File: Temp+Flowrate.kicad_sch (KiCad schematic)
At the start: 19 parts, among them Q7 PMOS, Q8 BUK6M61-60PX, U3 TLV9002QDRQ1

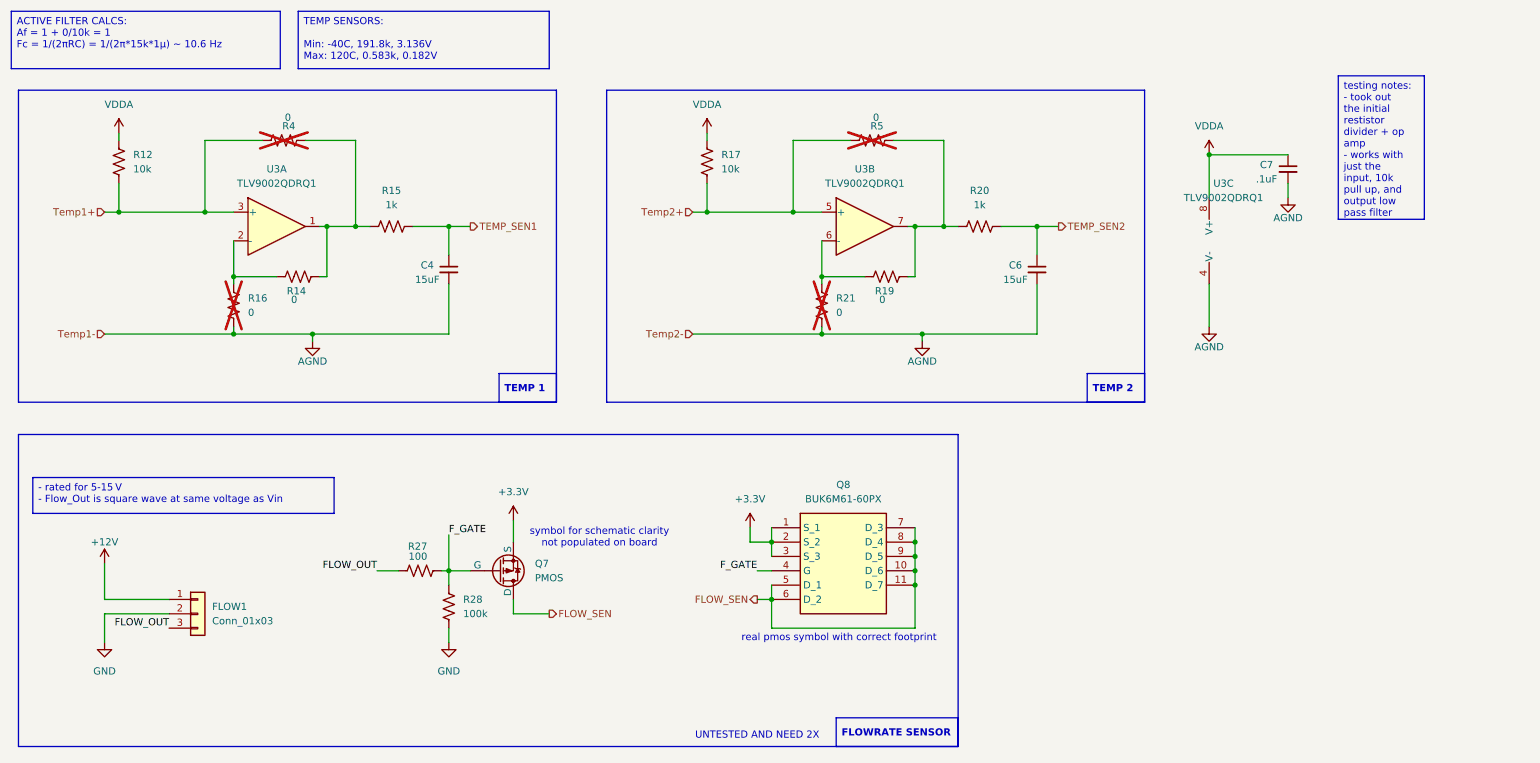
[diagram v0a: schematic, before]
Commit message: schem review changes
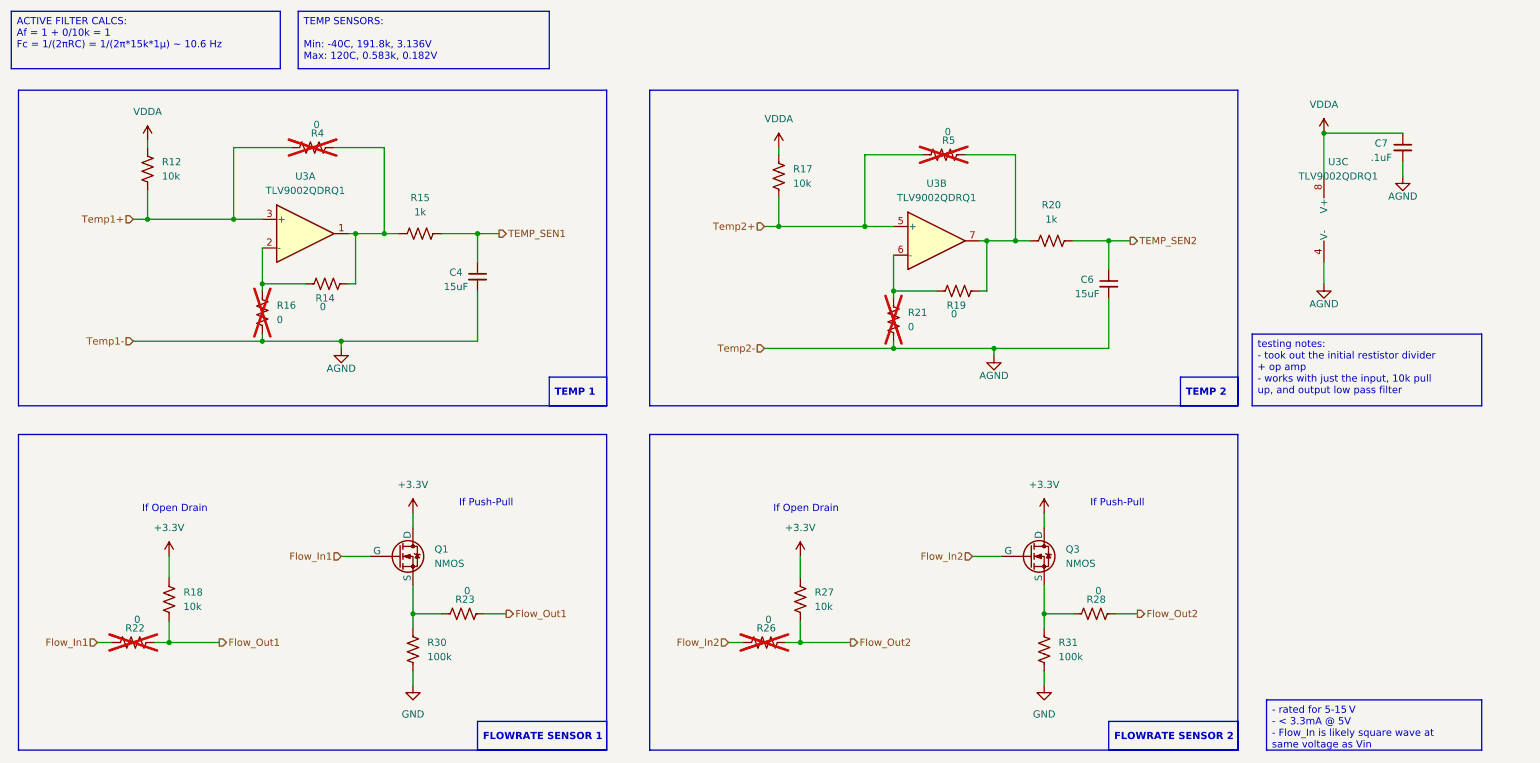
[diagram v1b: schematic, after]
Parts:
- removed FLOW1: Conn_01x03, Connector_Molex:Molex_Nano-Fit_105309-xx03_1x03_P2.50mm_Vertical, symbol Connector_Generic:Conn_01x03
- removed Q7: PMOS, symbol Simulation_SPICE:PMOS
- removed Q8: BUK6M61-60PX, BUK9M34100EX, symbol BUK6M61-60PX:BUK6M61-60PX
- added Q1, Q3: NMOS, IRLML0030TRPBF, symbol Simulation_SPICE:NMOS
- added R18: 10k, Resistor_SMD:R_0603_1608Metric, symbol Device:R_US
- added R22, R23, R26: 0, Resistor_SMD:R_0603_1608Metric, symbol Device:R_US
- added R30, R31: 100k, Resistor_SMD:R_0603_1608Metric, symbol Device:R_US
- R27: value 100 -> 10k
- R28: value 100k -> 0
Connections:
- net FLOW_OUT is gone; now on net +3.3V: R27.1
- net +3.3V: now also Q1.3 (D), Q3.3 (D), R18.1
- net GND: now also R30.2, R31.2; no longer R28.2
- net F_GATE: no longer names the net of R28.1
- net F_GATE: now also Q3.2 (S), R31.1; no longer R27.2
- new net: Q1.2 (S), R23.1, R30.1
- new net Flow_In1: Q1.1 (G), R22.1
- new net Flow_In2: Q3.1 (G), R26.1
- new net Flow_Out1: R18.2, R22.2, R23.2
- new net Flow_Out2: R26.2, R27.2, R28.2
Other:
- note added: "If Open Drain"
- note added: "If Push-Pull"
- note removed: "UNTESTED AND NEED 2X"
- note removed: "real pmos symbol with correct footprint"
- note removed: "symbol for schematic clarity not populated on board"
- moved on the sheet: C4, C6, C7, R12, R14, R15, R16, R17, R19, R20, R21, R4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
